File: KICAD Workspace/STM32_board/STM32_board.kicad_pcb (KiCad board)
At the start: 2 copper layers, 154.9 x 133.4 mm, 19 parts, among them J1 Power connector, J2 High side connector, J3 Sensors connector, J4 LCD interface, J5 Low side connector, J6 3v3_out, J7 Joystick connector, U1 CD4050BE, U2 LM7805_TO220, U3 LP2950-3.3_TO92

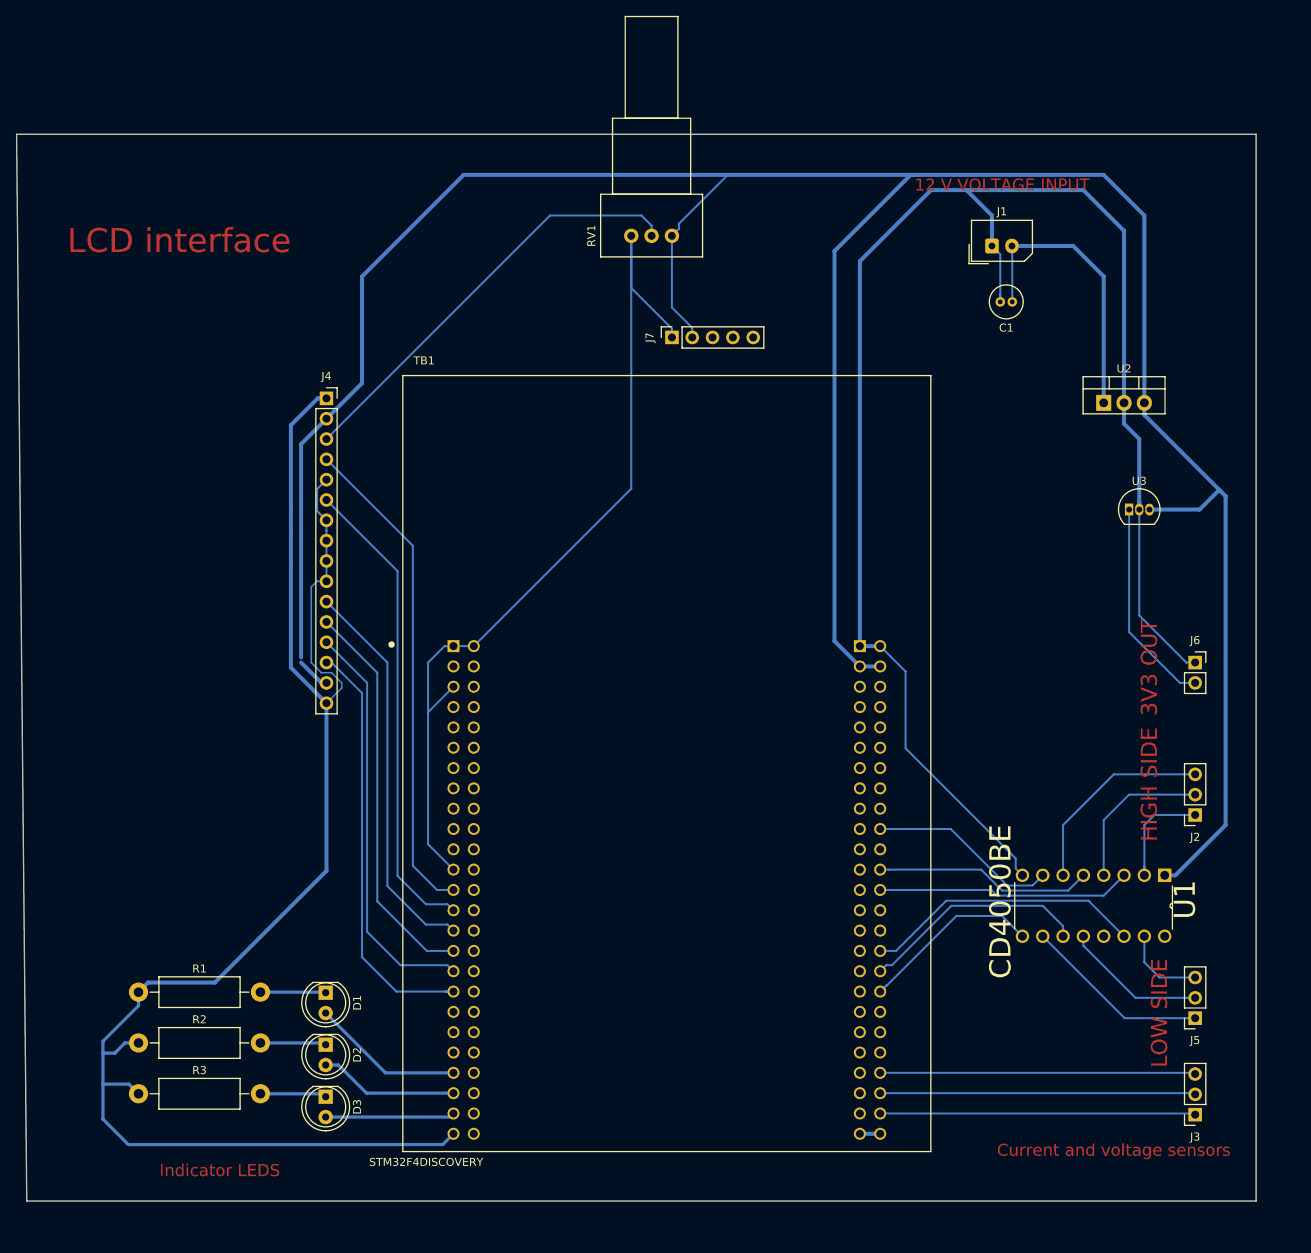
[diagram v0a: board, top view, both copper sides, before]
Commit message: Added some footprints.
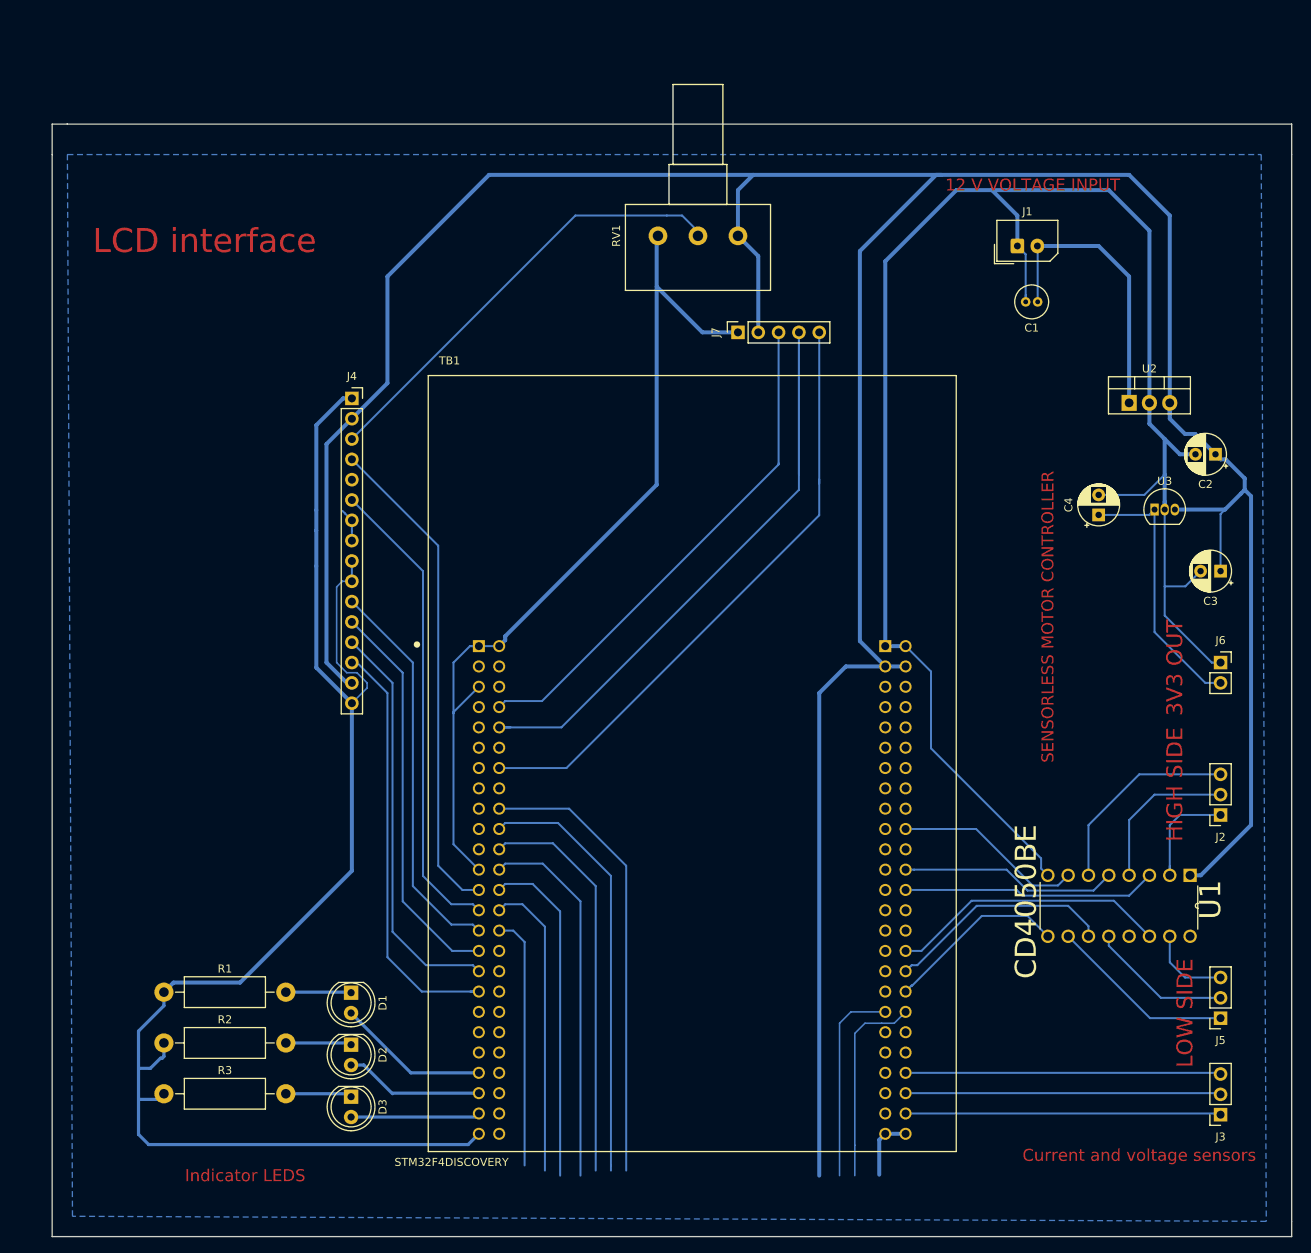
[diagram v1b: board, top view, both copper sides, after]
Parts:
- added C2: C, Capacitor_THT:CP_Radial_D5.0mm_P2.50mm, F.Cu at (199.4, 66.7)
- added C3: C3, Capacitor_THT:CP_Radial_D5.0mm_P2.50mm, F.Cu at (200.0, 81.3)
- added C4: C4, Capacitor_THT:CP_Radial_D5.0mm_P2.50mm, F.Cu at (184.8, 74.3)
- RV1: footprint Potentiometer_THT:Potentiometer_Vishay_248GJ-249GJ_Single_Horizontal -> Potentiometer_THT:Potentiometer_Alps_RK163_Single_Horizontal
- moved J7 8.28 mm to (139.7, 51.4)
- moved RV1 8.25 mm to (139.7, 39.4)
- moved D1 3.18 mm to (91.3, 134.0)
- moved D2 3.18 mm to (91.3, 140.5)
- moved D3 3.18 mm to (91.3, 147.0)
- moved J1 3.18 mm to (174.6, 40.6)
- moved J2 3.18 mm to (200.0, 111.8)
- moved J3 3.18 mm to (200.0, 149.2)
- moved J5 3.18 mm to (200.0, 137.2)
- moved J6 3.18 mm to (200.0, 92.7)
- moved TB1 3.18 mm to (134.0, 105.3)
- moved U1 3.18 mm to (178.4, 126.9)
- moved U2 3.18 mm to (188.6, 60.2)
- moved U3 3.18 mm to (191.8, 73.6)
- moved J4 3.17 mm to (91.4, 59.7)
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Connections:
- J7 pad 3: Net-(J7-Pad3) -> /JoystickADC1
- J7 pad 4: Net-(J7-Pad4) -> /JoystickADC2
- J7 pad 5: Net-(J7-Pad5) -> /JoystickButton
- TB1 pad P1_10: Net-(TB1-PadP1_10) -> /JoystickADC2
- TB1 pad P1_11: /JoystickButton -> Net-(TB1-PadP1_11)
- TB1 pad P1_14: Net-(TB1-PadP1_14) -> /JoystickButton
- TB1 pad P1_7: /JoystickADC1 -> Net-(TB1-PadP1_7)
- TB1 pad P1_8: Net-(TB1-PadP1_8) -> /JoystickADC1
- TB1 pad P1_9: /JoystickADC2 -> Net-(TB1-PadP1_9)
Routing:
- net /JoystickADC2: track 0.00 -> 88.7 mm
- net /5V: track 355.2 -> 436.4 mm
- net /JoystickButton: track 0.00 -> 76.4 mm
- net /JoystickADC1: track 0.00 -> 64.0 mm
- net Net-(TB1-PadP1_18): track 0.00 -> 56.9 mm
- net /GND: track 518.1 -> 572.5 mm
- net Net-(TB1-PadP1_20): track 0.00 -> 53.9 mm
- net Net-(TB1-PadP1_22): track 0.00 -> 50.2 mm
- net Net-(TB1-PadP1_24): track 0.00 -> 46.7 mm
- net Net-(TB1-PadP1_26): track 0.00 -> 42.4 mm
- net Net-(TB1-PadP1_28): track 0.00 -> 37.7 mm
- net Net-(TB1-PadP1_30): track 0.00 -> 31.7 mm
- net Net-(TB1-PadP2_37): track 0.00 -> 25.4 mm
- net Net-(TB1-PadP2_38): track 0.00 -> 25.2 mm
- net /3V3: track 26.2 -> 33.5 mm
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- added copper zone on B.Cu, net /GND
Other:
- board size 154.9 x 133.4 mm -> 154.9 x 139.1 mm
- board text added: "SENSORLESS MOTOR CONTROLLER"
